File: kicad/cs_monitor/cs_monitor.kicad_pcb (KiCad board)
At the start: 2 copper layers, 60.9 x 44.9 mm, 130 parts, among them J1 Conn_01x01_Female, J2 Conn_01x01_Female, J3 Conn_01x01_Female, J4 Conn, J5 Conn_01x01_Female, J6 Conn_01x01_Female, J7 Conn_01x01_Female, J8 Conn_01x01_Female, J9 Conn_01x01_Female, Q1 5N10, Q2 Q_NMOS_GSD, T1 HY931147C, U1 W5500, U2 OPA354AIDBVR, U3 LM2733XMF, U4 LMR50410XDBVR, U5 NCP1117-3.3, U6 MCP1700x, Y1 25MHz, Y2 16

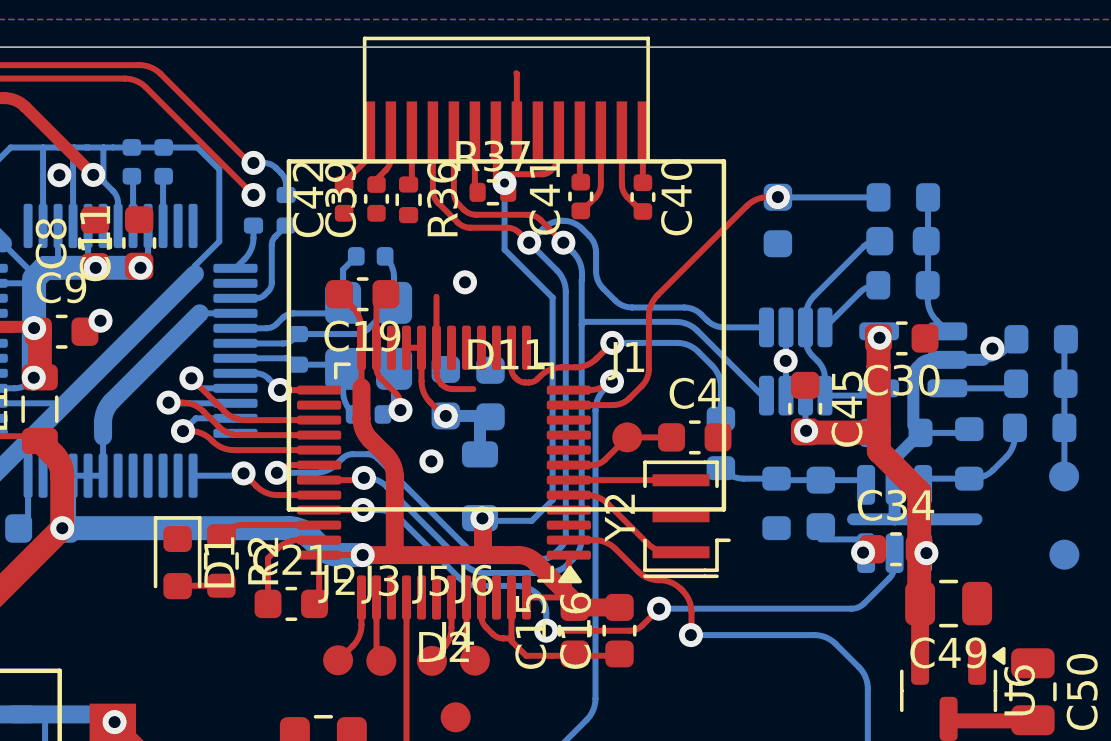
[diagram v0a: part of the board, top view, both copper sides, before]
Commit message: новый файл:    Documents/Rad.png 	изменено:      GNUPlot/alpha-01072025.dat 	изменено:      GNUPlot/mainChart-1.gp 	удалено:       kicad/cs_monitor/_autosave-cs_monitor.kicad_pcb 	удалено:       kicad/cs_monitor/cs_monitor-backups/cs_monitor-2025-07-07_163544.zip 	удалено:       kicad/cs_monitor/cs_monitor-backups/cs_monitor-2025-07-07_171133.zip 	изменено:      kicad/cs_monitor/cs_monitor.kicad_pcb 	изменено:      kicad/cs_monitor/cs_monitor.kicad_prl 	изменено:      kicad/cs_monitor/cs_monitor.kicad_pro 	удалено:       kicad/cs_monitor/~_autosave-cs_monitor.kicad_pcb.lck 	удалено:       kicad/cs_monitor/~cs_monitor.kicad_sch.lck
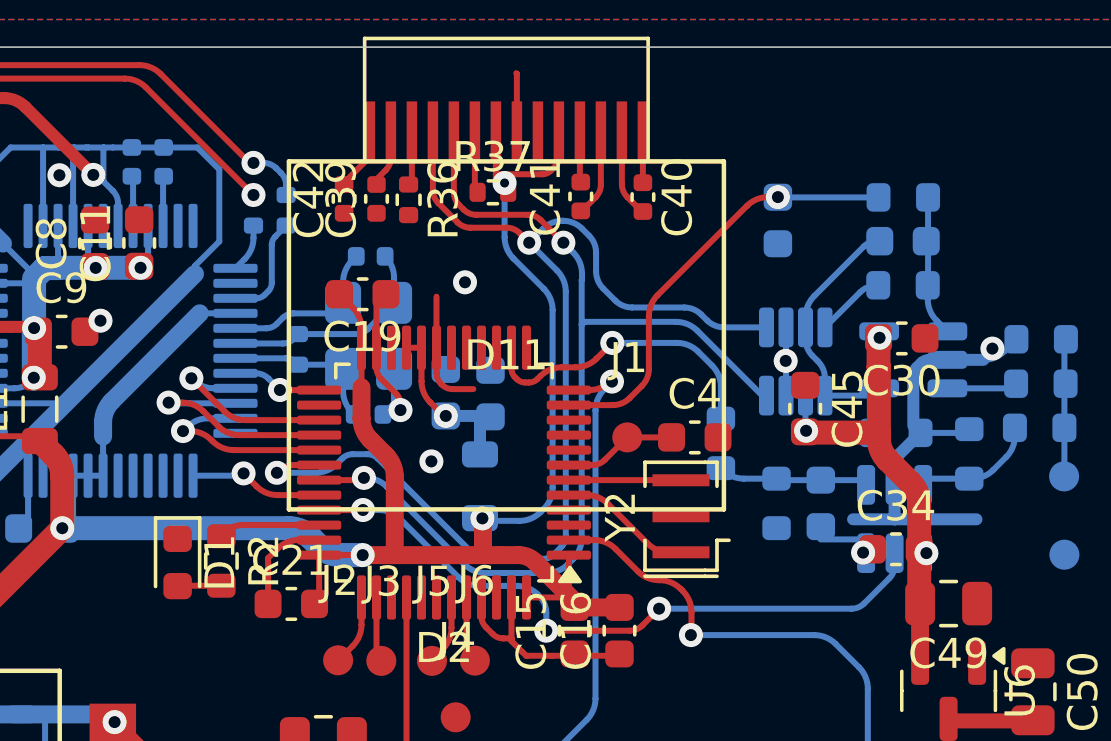
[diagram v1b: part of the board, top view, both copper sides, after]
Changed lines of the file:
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@@
 		(sheetname "/")
 		(sheetfile "cs_monitor.kicad_sch")
+		(clearance 0.15)
 		(attr smd)
 		(fp_line
@@
 	(segment
 		(start 111.24625 49.24625)
-		(end 111.24625 48.13625)
+		(end 111.24625 48.550464)
 		(width 0.2)
 		(layer "B.Cu")
@@
 	)
 	(segment
-		(start 111.24625 48.13625)
+		(start 111.539143 47.843357)
 		(end 111.68625 47.69625)
 		(width 0.2)
@@
 	)
 	(arc
+		(start 111.24625 48.550464)
+		(mid 111.32237 48.167781)
+		(end 111.539143 47.843357)
+		(width 0.2)
+		(layer "B.Cu")
+		(net 2)
+	)
+	(arc
 		(start 81.567157 76.782843)
 		(mid 81.480448 76.912612)
@@
 	)
 	(segment
-		(start 118.23 49.07)
-		(end 118.23 55.82)
+		(start 118.23 49.484214)
+		(end 118.23 55.405786)
 		(width 0.2)
 		(layer "B.Cu")
@@
 	(segment
 		(start 116.63 45.25)
-		(end 116.63 47.47)
+		(end 116.63 47.055786)
 		(width 0.2)
 		(layer "B.Cu")
@@
 	)
 	(segment
-		(start 116.63 47.47)
-		(end 118.23 49.07)
+		(start 116.922893 47.762893)
+		(end 117.937107 48.777107)
 		(width 0.2)
 		(layer "B.Cu")
@@
 	)
 	(segment
-		(start 118.23 55.82)
-		(end 117.5375 56.5125)
+		(start 117.937107 56.112893)
+		(end 117.830393 56.219607)
 		(width 0.2)
 		(layer "B.Cu")
@@
 	)
 	(segment
-		(start 117.5375 56.5125)
+		(start 117.123286 56.5125)
 		(end 116.44 56.5125)
 		(width 0.2)
@@
 	)
 	(arc
+		(start 118.23 55.405786)
+		(mid 118.15388 55.788469)
+		(end 117.937107 56.112893)
+		(width 0.2)
+		(layer "B.Cu")
+		(net 8)
+	)
+	(arc
 		(start 103.539143 52.523357)
 		(mid 103.32237 52.84778)
@@
 	)
 	(arc
+		(start 117.830393 56.219607)
+		(mid 117.50597 56.43638)
+		(end 117.123286 56.5125)
+		(width 0.2)
+		(layer "B.Cu")
+		(net 8)
+	)
+	(arc
+		(start 118.23 49.484214)
+		(mid 118.15388 49.101531)
+		(end 117.937107 48.777107)
+		(width 0.2)
+		(layer "B.Cu")
+		(net 8)
+	)
+	(arc
 		(start 80.94625 50.570464)
 		(mid 80.87013 50.187781)
@@
 		(net 8)
 	)
+	(arc
+		(start 116.63 47.055786)
+		(mid 116.70612 47.438469)
+		(end 116.922893 47.762893)
+		(width 0.2)
+		(layer "B.Cu")
+		(net 8)
+	)
 	(segment
 		(start 97.47 44.38625)
@@
 	)
 	(segment
-		(start 106.33625 53.09375)
+		(start 106.043357 53.386643)
 		(end 105.91 53.52)
 		(width 0.2)
@@
 	(segment
 		(start 107.65875 53.09375)
-		(end 106.33625 53.09375)
+		(end 106.750464 53.09375)
+		(width 0.2)
+		(layer "B.Cu")
+		(net 55)
+	)
+	(arc
+		(start 106.043357 53.386643)
+		(mid 106.36778 53.16987)
+		(end 106.750464 53.09375)
 		(width 0.2)
 		(layer "B.Cu")
@@
 	)
 	(segment
-		(start 106.52375 52.09375)
+		(start 106.230857 51.800857)
 		(end 106.19 51.76)
 		(width 0.2)
@@
 	(segment
 		(start 107.65875 52.09375)
-		(end 106.52375 52.09375)
+		(end 106.937964 52.09375)
+		(width 0.2)
+		(layer "B.Cu")
+		(net 58)
+	)
+	(arc
+		(start 106.230857 51.800857)
+		(mid 106.55528 52.01763)
+		(end 106.937964 52.09375)
 		(width 0.2)
 		(layer "B.Cu")
@@
 	(segment
 		(start 129.105 53.57)
-		(end 129.105 54.185)
+		(end 129.105 53.770786)
 		(width 0.8)
 		(layer "F.Cu")
@@
 	)
 	(segment
-		(start 130.45 55.53)
+		(start 130.45 55.944214)
 		(end 130.45 57.46)
 		(width 0.8)
@@
 	)
 	(segment
-		(start 129.105 54.185)
-		(end 130.45 55.53)
+		(start 129.397893 54.477893)
+		(end 130.157107 55.237107)
 		(width 0.8)
 		(layer "F.Cu")
@@
 		(net 117)
 	)
+	(arc
+		(start 129.105 53.770786)
+		(mid 129.18112 54.153469)
+		(end 129.397893 54.477893)
+		(width 0.8)
+		(layer "F.Cu")
+		(net 117)
+	)
+	(arc
+		(start 130.45 55.944214)
+		(mid 130.37388 55.561531)
+		(end 130.157107 55.237107)
+		(width 0.8)
+		(layer "F.Cu")
+		(net 117)
+	)
